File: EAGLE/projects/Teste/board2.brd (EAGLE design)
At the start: 100 x 80 mm, 21 parts, among them IC1 317T, IC2 7805T

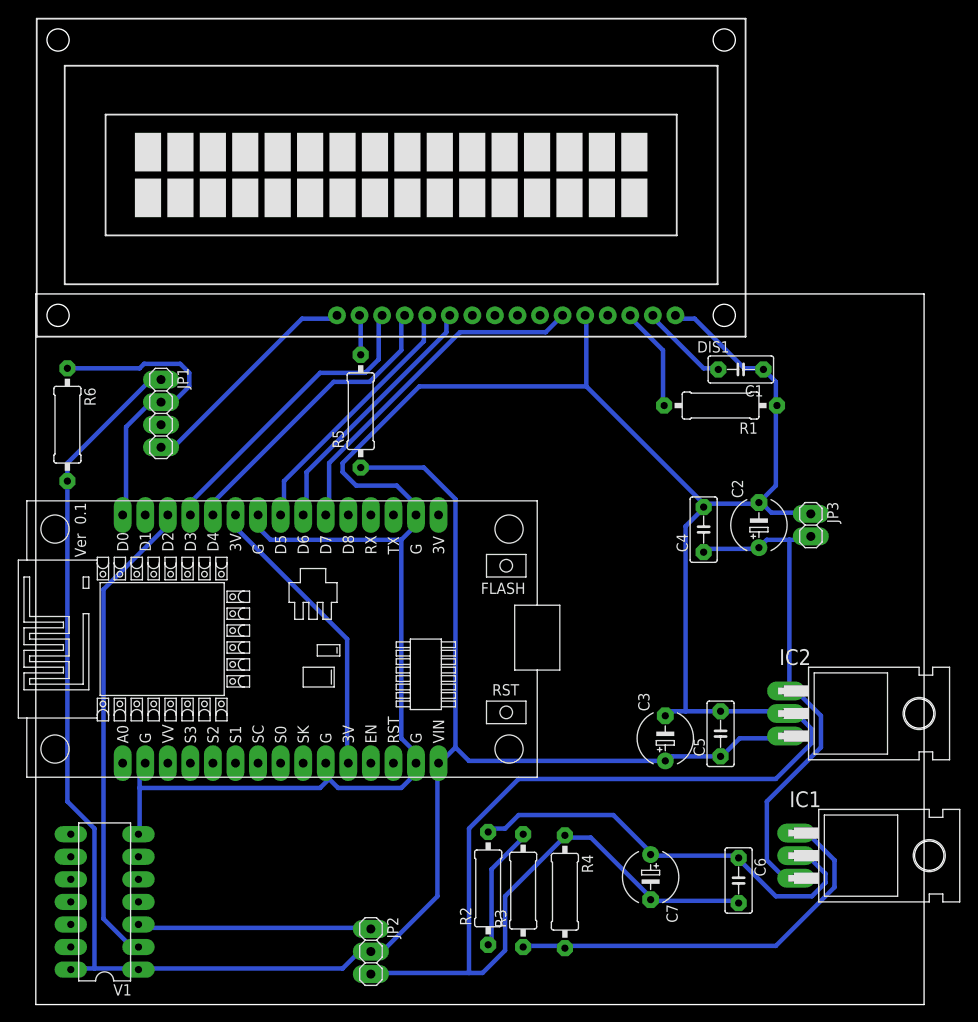
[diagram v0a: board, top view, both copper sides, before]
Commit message: Placa Roteada
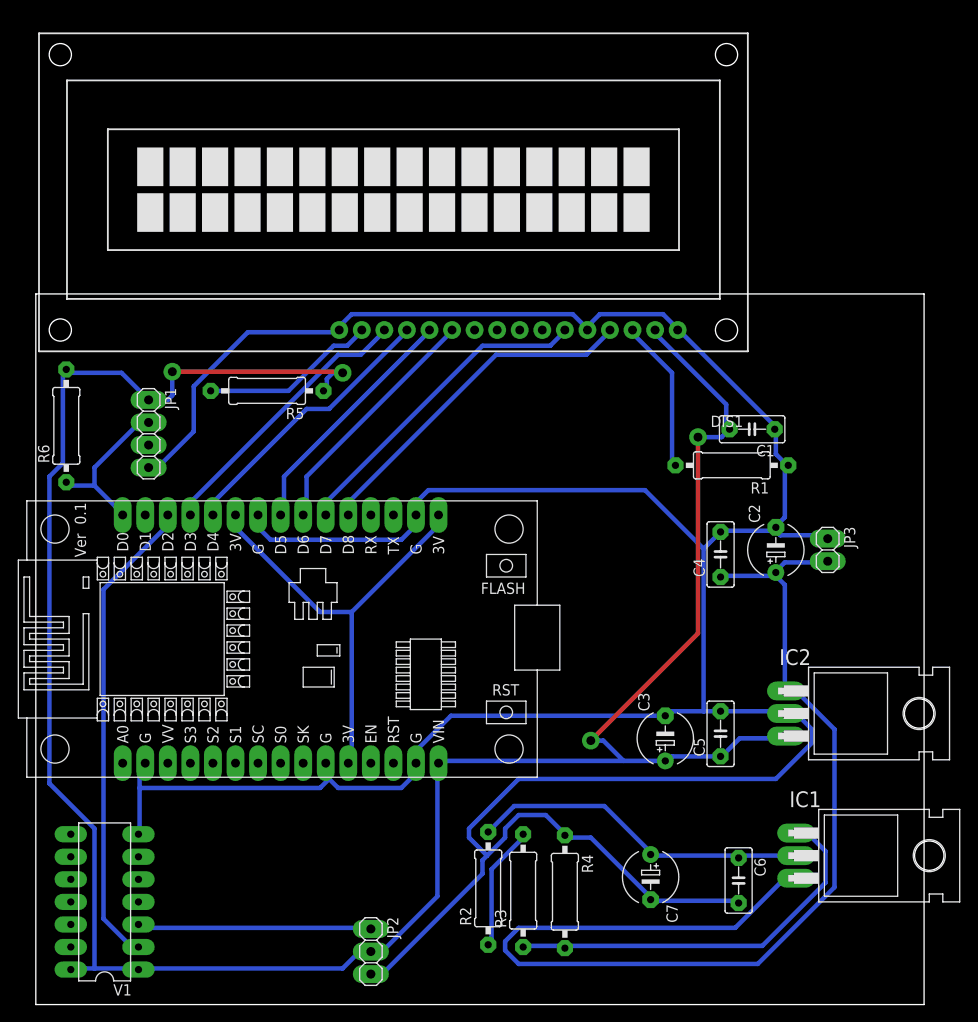
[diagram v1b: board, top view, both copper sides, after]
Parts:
- moved R5 10.8 mm to (26.0, 69.1), turned to 180 degrees
- moved C1 6.85 mm to (80.6, 64.8)
- moved R1 6.85 mm to (78.4, 60.7)
- moved C2 3.38 mm to (83.3, 51.2)
- moved JP3 3.38 mm to (89.2, 51.2)
- moved C4 3.38 mm to (77.1, 50.7)
- moved JP1 2.68 mm to (12.7, 64.3)
- moved DIS1 1.67 mm to (40.3, 91.4)
- moved R6 0.18 mm to (3.43, 65.2), turned to 90 degrees
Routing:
- net N$3: track 58.2 -> 129.5 mm
- net +5V: track 224.2 -> 272.5 mm, vias 0 -> 4
- net LCD_RS: track 0.00 -> 39.0 mm
- net 3V: track 33.2 -> 50.6 mm
- net DATA_DHT: track 35.0 -> 18.3 mm
- net N$6: track 4.46 -> 19.9 mm
- net +3V3: track 48.4 -> 38.5 mm
- net N$1: track 11.7 -> 17.4 mm
- net LCD_D7: track 34.4 -> 31.4 mm
- net GND: track 387.3 -> 390.2 mm
- net LCD_E: track 39.2 -> 36.5 mm
- net LCD_D6: track 33.8 -> 31.4 mm
- net N$5: track 46.8 -> 45.0 mm
- net LCD_D4: track 29.4 -> 27.8 mm
- net LCD_D5: track 29.4 -> 27.8 mm
